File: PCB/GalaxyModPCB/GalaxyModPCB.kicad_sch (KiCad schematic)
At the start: 55 parts, among them J1 Power Header, J2 Boot mode, J3 LED RGBW Connector, J4 JTAG, J5 USB to UART, J6 Motor Connector, J7 Projector Connector, Q1 BC817-40-7-F, Q2 BC817-40-7-F, Q3 BC817-40-7-F, Q4 BC817-40-7-F, Q5 BC817-40-7-F, Q6 BC817-40-7-F, SW1 Motor, SW2 Brightness, SW3 Colour, SW4 On/Off, U1 AMS1117-3.3, U2 ESP32-WROOM-32

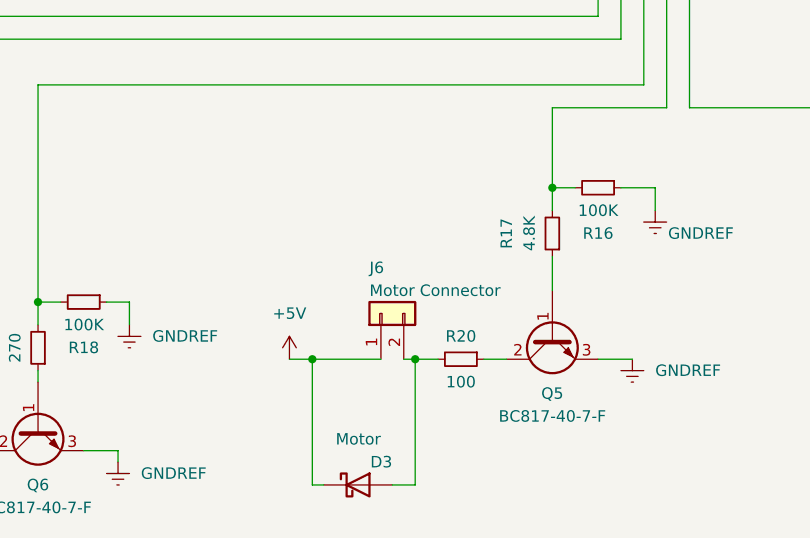
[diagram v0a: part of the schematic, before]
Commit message: icy layout suggestions
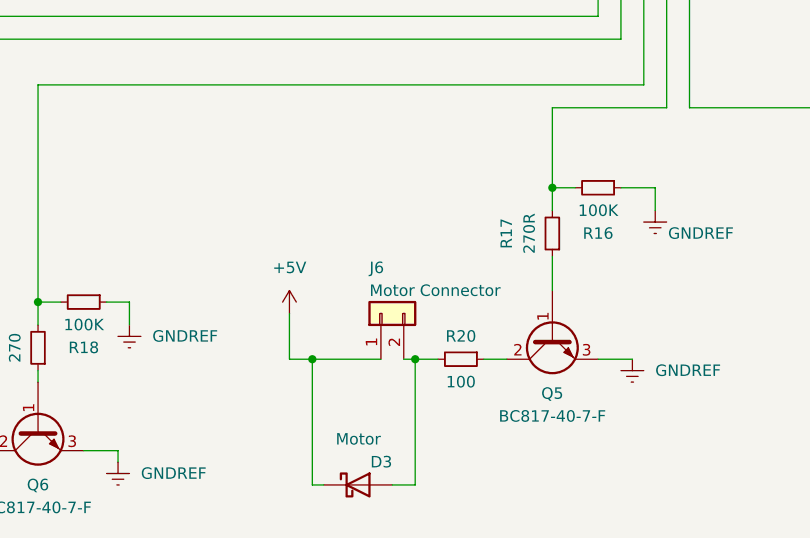
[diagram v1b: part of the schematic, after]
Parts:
- J2: footprint Jumper:SolderJumper-2_P1.3mm_Open_TrianglePad1.0x1.5mm -> Resistor_SMD:R_0805_2012Metric_Pad1.20x1.40mm_HandSolder
- R17: value 4.8K -> 270R
